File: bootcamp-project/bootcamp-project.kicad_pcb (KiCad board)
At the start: 2 copper layers, 17 parts, among them J3 FTDI, SW1 SW_Push, U1 ATmega328P-A, Y1 16MHz

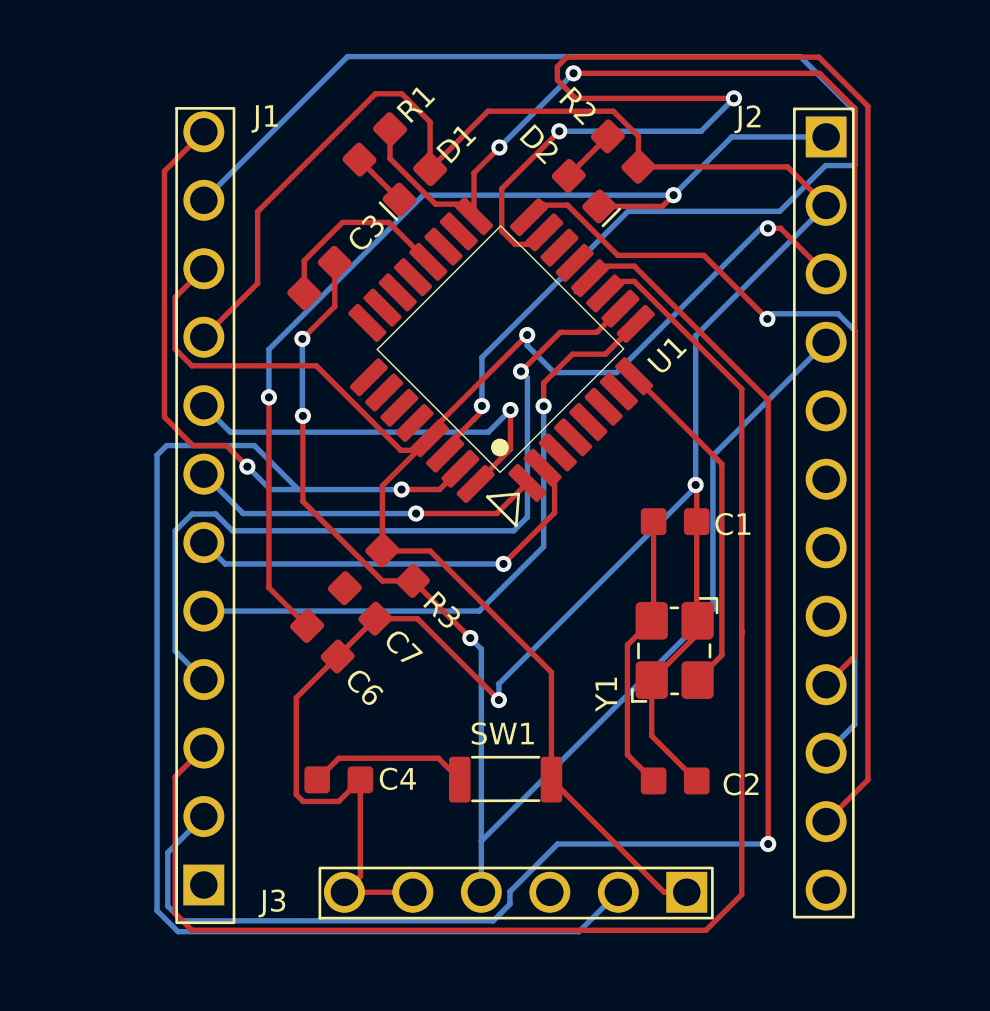
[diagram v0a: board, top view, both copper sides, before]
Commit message: pcb: new try, again
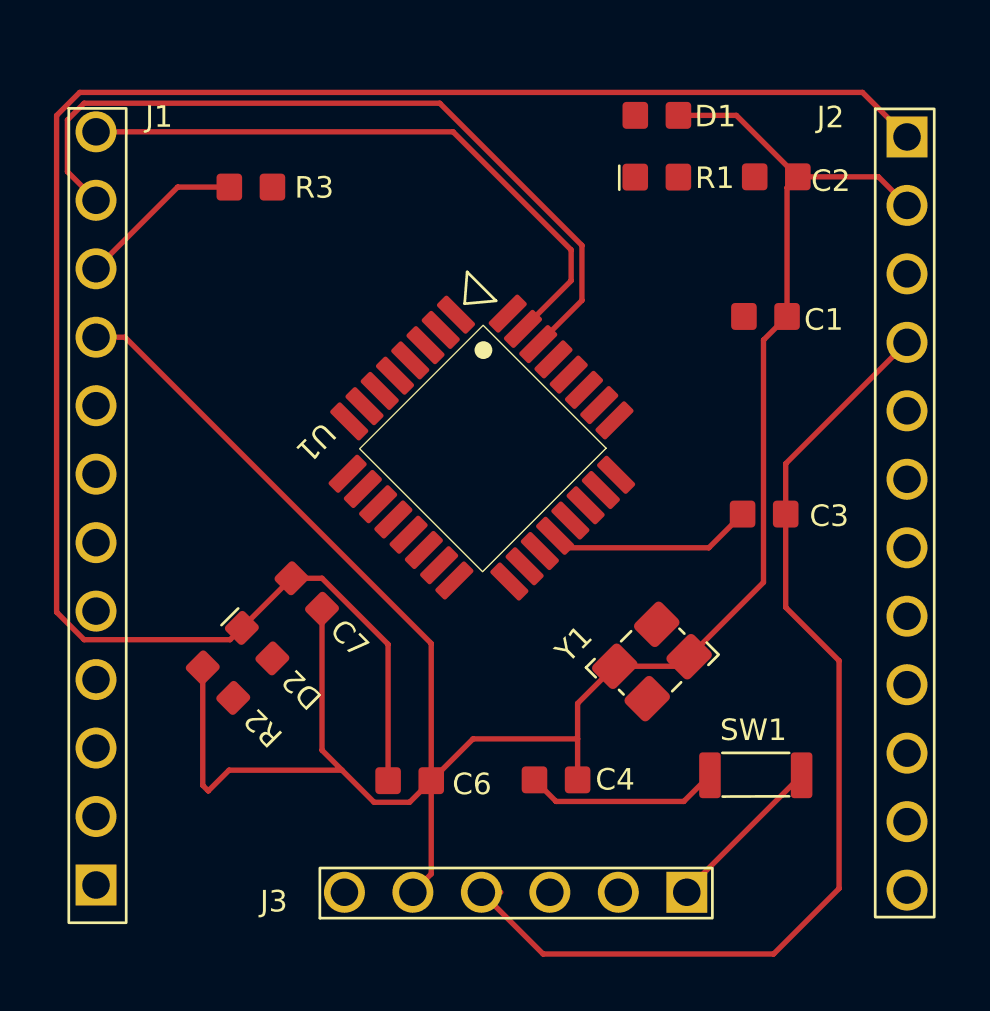
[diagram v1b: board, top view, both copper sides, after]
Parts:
- moved R2 24.8 mm to (99.6, 97.5), turned to 135 degrees
- moved C2 22.7 mm to (120.3, 78.7)
- moved D2 20.8 mm to (101.0, 96.1), turned to 135 degrees
- moved C3 18.7 mm to (119.8, 91.2), turned to 0 degrees
- moved R3 15.1 mm to (100.8, 79.1), turned to 0 degrees
- moved R1 10.5 mm to (115.8, 78.8), turned to 0 degrees
- moved D1 9.36 mm to (115.8, 76.4), turned to 0 degrees
- moved SW1 9.28 mm to (119.5, 101.0)
- moved C1 8.31 mm to (119.9, 83.9)
- moved C4 8.06 mm to (112.1, 101.1)
- moved C6 6.10 mm to (106.7, 101.1), turned to 0 degrees
- moved J1 4.00 mm to (95.0, 91.2)
- moved U1 3.61 mm to (109.4, 88.8), turned to -135 degrees
- moved J2 3.00 mm to (125.0, 92.5)
- moved C7 2.01 mm to (102.9, 94.2)
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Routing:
- net MOSI: track 60.5 -> 0.00 mm, vias 2 -> 0
- net D7: track 54.2 -> 0.00 mm
- net D8: track 53.9 -> 0.00 mm, vias 1 -> 0
- net DTR: track 58.5 -> 12.3 mm, vias 2 -> 0
- net SCK: track 44.7 -> 0.00 mm, vias 2 -> 0
- net TXO: track 64.6 -> 23.1 mm, vias 2 -> 0
- net RAW: track 37.7 -> 70.7 mm, vias 2 -> 0
- net MISO: track 31.2 -> 0.00 mm, vias 1 -> 0
- net D6: track 29.9 -> 0.00 mm, vias 1 -> 0
- net D5: track 24.0 -> 0.00 mm, vias 1 -> 0
- net RXI: track 50.1 -> 29.3 mm, vias 1 -> 0
- net D4: track 16.0 -> 0.00 mm, vias 1 -> 0
- net D2: track 15.4 -> 0.00 mm, vias 1 -> 0
- net D3: track 13.1 -> 0.00 mm, vias 1 -> 0
- net Net-(U1-XTAL2/PB7): track 13.0 -> 0.00 mm
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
